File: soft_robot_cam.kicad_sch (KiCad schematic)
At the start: 85 parts, among them J1 Connector, J10 Screw_Terminal_01x02, J11 Conn_02x02_Counter_Clockwise, J2 Conn_01x06, J3 Conn_01x03, J4 Conn_01x05_Pin, J5 Conn_01x02_Pin, J6 Screw_Terminal_01x02, J7 Screw_Terminal_01x02, J8 Conn_01x24_Socket, J9 Screw_Terminal_01x02, Q1 S8050, Q2 S8050, Q3 AO3401A, Q4 AO3400A, SW4 SW_DIP_x02, U12 XC6206P282MR, U13 XC6206P122MR, U14 SY8113IADC, U3 MPU6500, U4 DRV8874PWPR, U5 DRV8874PWPR, U9 ESP32-S3-WROOM-1-N16R8

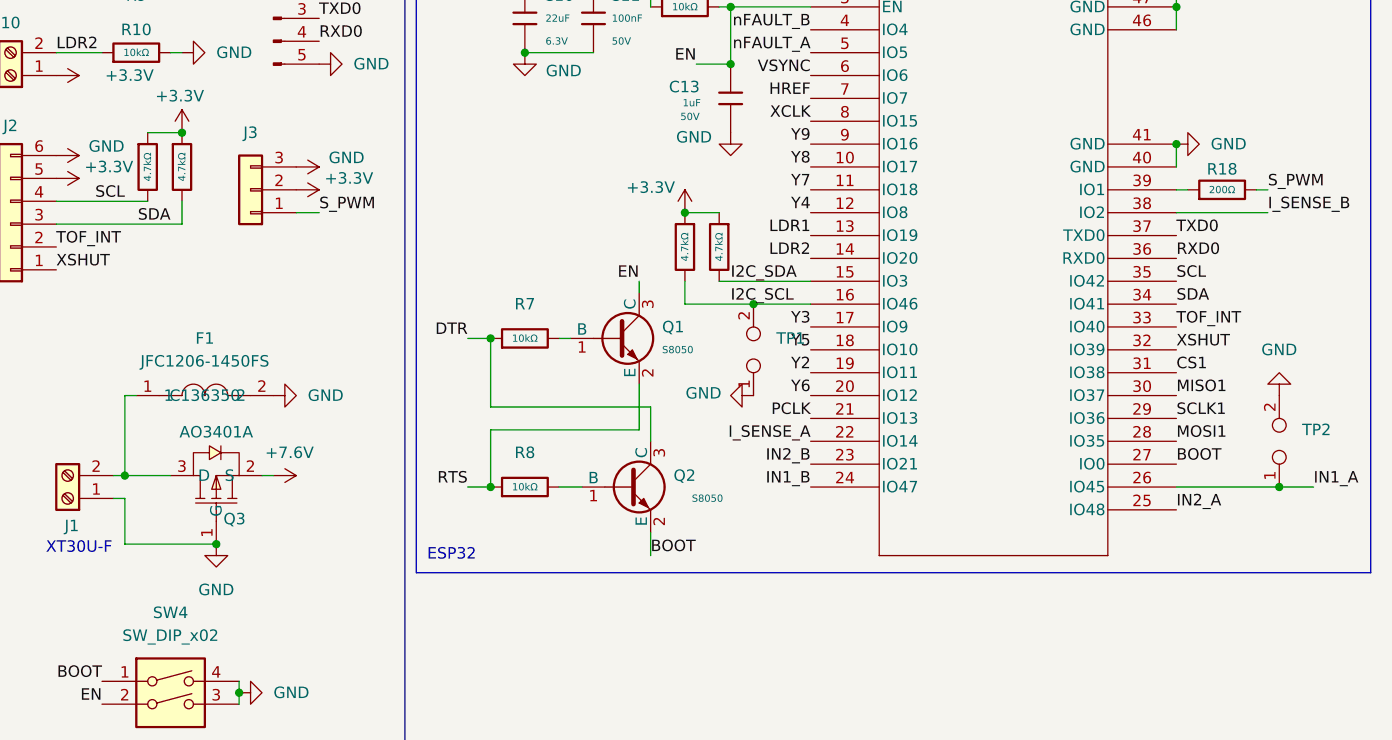
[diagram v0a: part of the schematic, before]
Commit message: Minor Changes
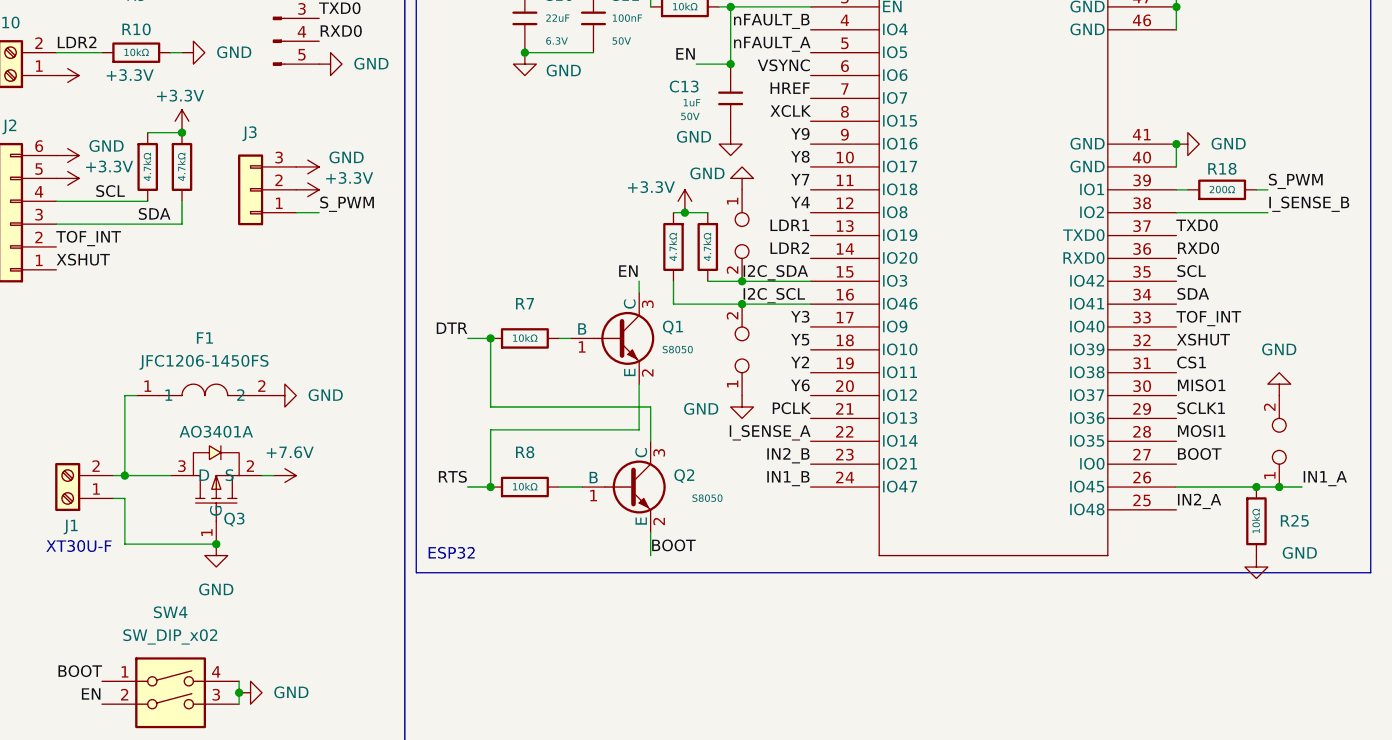
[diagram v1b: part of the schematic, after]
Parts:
- added R25: 10kΩ, PCM_JLCPCB:R_0603, symbol PCM_JLCPCB-Resistors:0603,10kΩ
- added TP3: TestPoint_2Pole, symbol Connector:TestPoint_2Pole
- F1: LCSC C136350 -> (none); LCSC Part C136350 -> C41367230
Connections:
- net GND: now also R25.2, TP3.1
- net I2C_SDA: now also TP3.2
- net IN1_A: now also R25.1
